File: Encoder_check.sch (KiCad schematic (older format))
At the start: 18 parts, among them J1 Conn_01x08, J2 Conn_01x06, P1 Digital, P2 Analog, P3 CONN_01X01, P4 CONN_01X01, P5 CONN_01X01, P6 CONN_01X01, U1 AM26LV32xD, U2 ST490AB

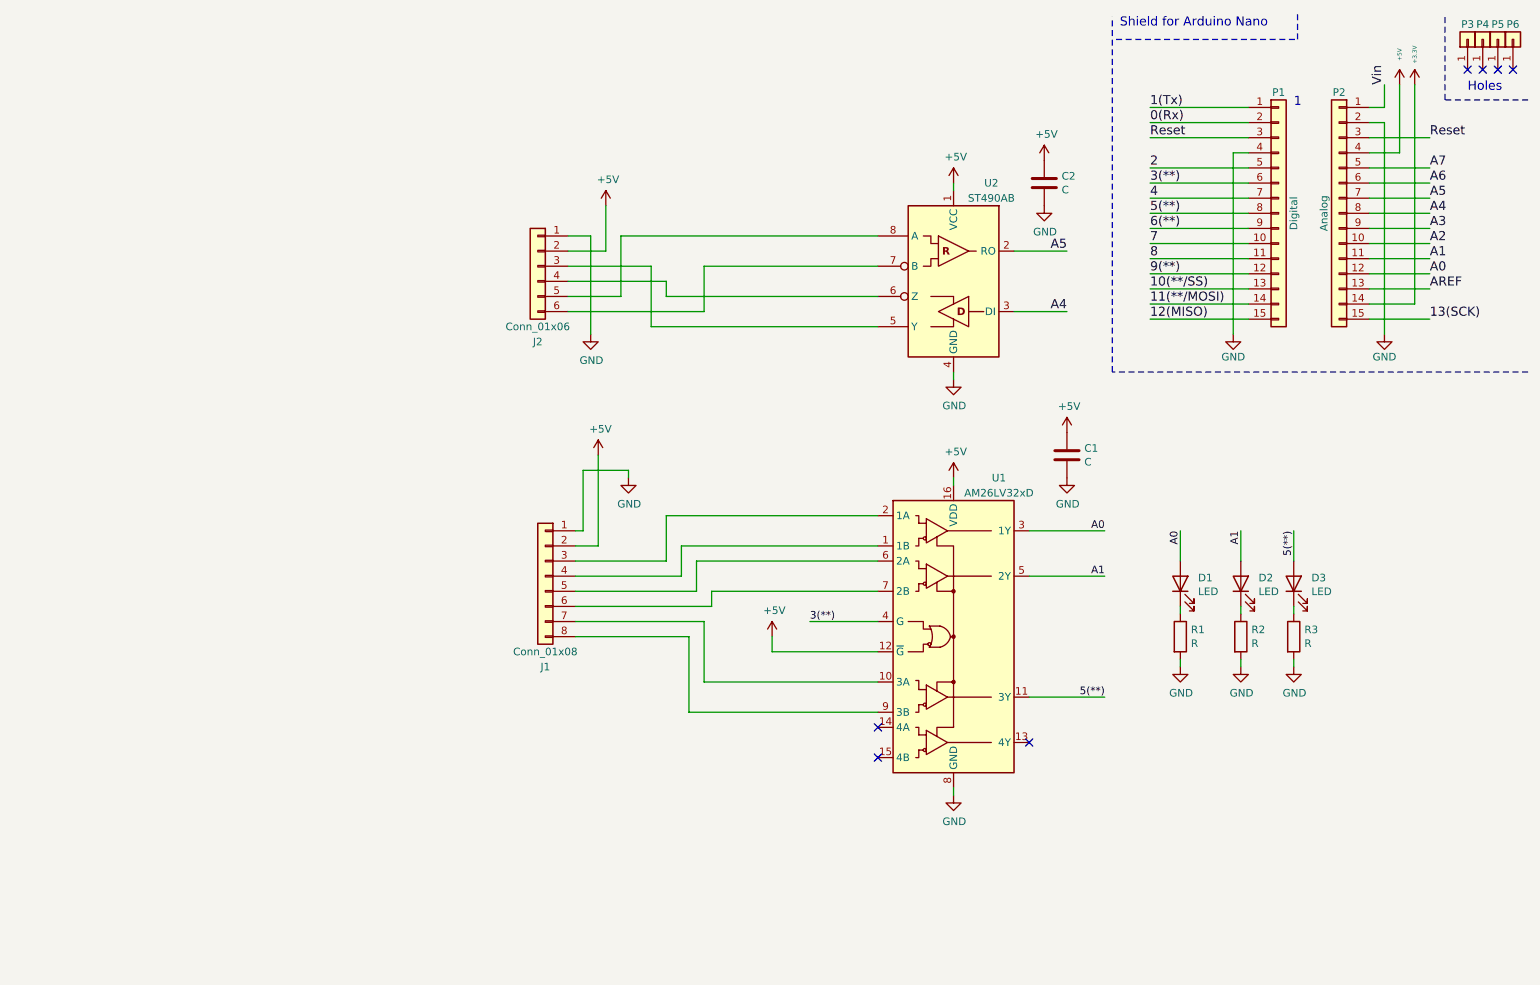
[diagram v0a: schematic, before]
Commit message: AW
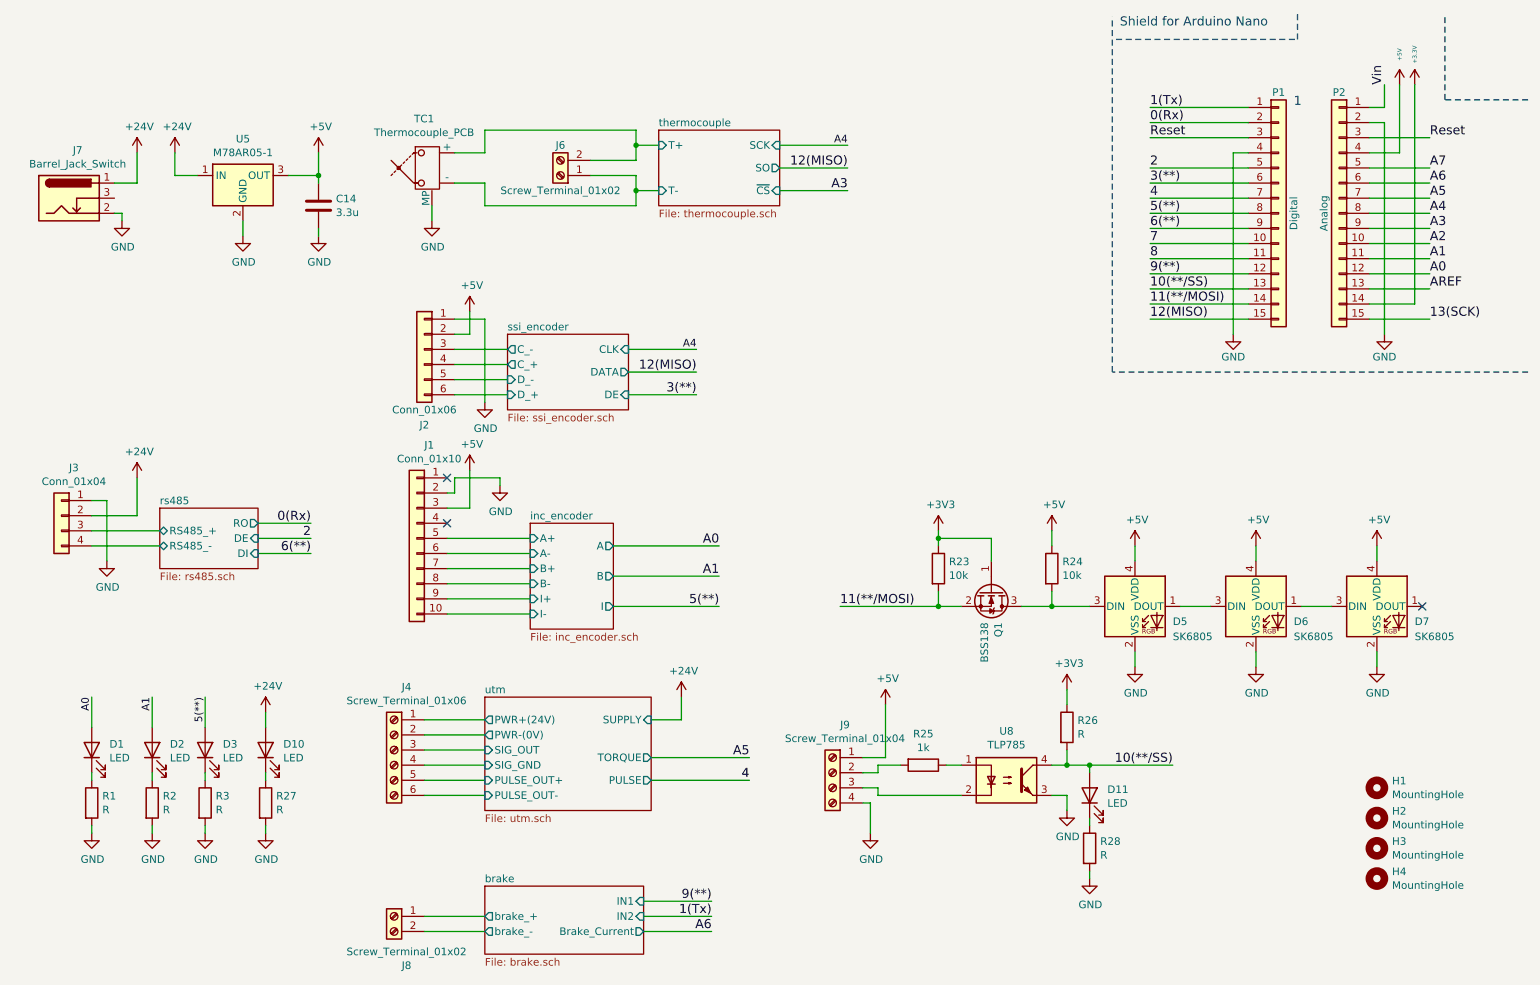
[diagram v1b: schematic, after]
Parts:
- removed C1, C2: C, Capacitor_SMD:C_0603_1608Metric, symbol Device:C
- removed J1: Conn_01x08, TerminalBlock_TE-Connectivity:TerminalBlock_TE_282834-8_1x08_P2.54mm_Horizontal, symbol Connector_Generic:Conn_01x08
- removed P3, P4, P5, P6: CONN_01X01, Socket_Arduino_Nano:1pin_Nano, symbol Connector_Generic:Conn_01x01
- removed U1: AM26LV32xD, Package_SO:SOIC-16_3.9x9.9mm_P1.27mm, symbol Interface:AM26LV32xD
- removed U2: ST490AB, Package_SO:SO-8_3.9x4.9mm_P1.27mm, symbol mylib:ST490AB
- added C14: 3.3u, Capacitor_SMD:C_0805_2012Metric, symbol Device:C
- added D10, D11: LED, LED_SMD:LED_0603_1608Metric, symbol Device:LED
- added D5, D6, D7: SK6805, LED_SMD:LED_SK6805_PLCC4_2.4x2.7mm_P1.3mm, symbol LED:SK6805
- added H1, H2, H3, H4: MountingHole, MountingHole:MountingHole_3.2mm_M3, symbol Mechanical:MountingHole
- added J1: Conn_01x10, Connector_Multicomp:Multicomp_MC9A12-1034_2x05_P2.54mm_Vertical, symbol Connector_Generic:Conn_01x10
- added J3: Conn_01x04, Connector_JST:JST_EH_S4B-EH_1x04_P2.50mm_Horizontal, symbol Connector_Generic:Conn_01x04
- added J4: Screw_Terminal_01x06, TerminalBlock_TE-Connectivity:TerminalBlock_TE_282834-6_1x06_P2.54mm_Horizontal, symbol Connector:Screw_Terminal_01x06
- added J6, J8: Screw_Terminal_01x02, TerminalBlock_Phoenix:TerminalBlock_Phoenix_MKDS-1,5-2-5.08_1x02_P5.08mm_Horizontal, symbol Connector:Screw_Terminal_01x02
- added J7: Barrel_Jack_Switch, Connector_BarrelJack:BarrelJack_Horizontal, symbol Connector:Barrel_Jack_Switch
- added J9: Screw_Terminal_01x04, TerminalBlock_TE-Connectivity:TerminalBlock_TE_282834-4_1x04_P2.54mm_Horizontal, symbol Connector:Screw_Terminal_01x04
- added Q1: BSS138, Package_TO_SOT_SMD:SOT-23, symbol Transistor_FET:BSS138
- added R23, R24: 10k, Resistor_SMD:R_0603_1608Metric, symbol Device:R
- added R25: 1k, Resistor_SMD:R_0603_1608Metric, symbol Device:R
- added R26, R27, R28: R, Resistor_SMD:R_0603_1608Metric, symbol Device:R
- added TC1: Thermocouple_PCB, Connector_Omega:Omega_PCC-SMP_1x2_P13.70mm_Horizontal, symbol mylib:Thermocouple_PCB
- added U5: M78AR05-1, Converter_DCDC_my:Converter_DCDC_MINIMAX_M78AR05-1_THT, symbol mylib:M78AR05-1
- added U8: TLP785, Package_DIP:DIP-4_W7.62mm, symbol Isolator:TLP785
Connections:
- net +3V3: now also Q1.1 (G), R23.1, R26.1
- net +5V: now also C14.1, D5.4 (VDD), D6.4 (VDD), D7.4 (VDD), J1.3 (Pin_3), J9.1 (Pin_1), R24.1, U5.3 (OUT)
- net 10(**/SS): now also D11.2 (A), R26.2, U8.4
- net 11(**/MOSI): now also Q1.2 (S), R23.2
- net GND: now also C14.2, D5.2 (VSS), D6.2 (VSS), D7.2 (VSS), J1.2 (Pin_2), J3.1 (Pin_1), J7.2, J9.4 (Pin_4), R27.2, R28.2, TC1.3 (MP), U5.2 (GND), U8.3
- net ssi_encoder/C_-: now reaches J2.3 (Pin_3)
- net ssi_encoder/C_+: now reaches J2.4 (Pin_4)
- net ssi_encoder/D_+: now reaches J2.6 (Pin_6)
- net ssi_encoder/D_-: now reaches J2.5 (Pin_5)
- new net: D5.1 (DOUT), D6.3 (DIN)
- new net: D5.3 (DIN), Q1.3 (D), R24.2
- new net: D6.1 (DOUT), D7.3 (DIN)
- new net: R25.1, U8.1
- new net: J9.3 (Pin_3), U8.2
- new net: J9.2 (Pin_2), R25.2
- new net: D10.1 (K), R27.1
- new net: D11.1 (K), R28.1
- new net +24V: D10.2 (A), J3.2 (Pin_2), J7.1, U5.1 (IN)
- new net brake/brake_+: J8.1 (Pin_1)
- new net brake/brake_-: J8.2 (Pin_2)
- new net inc_encoder/A+: J1.5 (Pin_5)
- new net inc_encoder/A-: J1.6 (Pin_6)
- new net inc_encoder/B+: J1.7 (Pin_7)
- new net inc_encoder/B-: J1.8 (Pin_8)
- new net inc_encoder/I+: J1.9 (Pin_9)
- new net inc_encoder/I-: J1.10 (Pin_10)
- new net rs485/RS485_+: J3.3 (Pin_3)
- new net rs485/RS485_-: J3.4 (Pin_4)
- new net thermocouple/T+: J6.2 (Pin_2), TC1.1 (+)
- new net thermocouple/T-: J6.1 (Pin_1), TC1.2 (-)
- new net utm/PULSE_OUT+: J4.5 (Pin_5)
- new net utm/PULSE_OUT-: J4.6 (Pin_6)
- new net utm/PWR+(24V): J4.1 (Pin_1)
- new net utm/PWR-(0V): J4.2 (Pin_2)
- new net utm/SIG_GND: J4.4 (Pin_4)
- new net utm/SIG_OUT: J4.3 (Pin_3)
- no-connect marks 7 -> 3
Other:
- note removed: "Holes"
- moved on the sheet: D1, D2, D3, R1, R2, R3
